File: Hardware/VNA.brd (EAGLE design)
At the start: 122 x 96 mm, 499 parts, among them IC1 ADL5801, IC10 LT5560, IC11 THS4521IDGKR, IC12 MCP33131D-10-E/MS, IC13 SI5351C, IC14 MAX2871, IC15 NCP702-3.3, IC16 RFSW6042, IC17 AP2114H, IC18 RFSW6042, IC19 MAX2871, IC2 LT5560, IC20 NCP702-3.3, IC21 AP2114H, IC22 QPC6324, IC23 RFSA3714, IC24 TRF37A73, IC25 QPC6324, IC26 QPC6324, IC27 QPC6324, IC28 LDL212PU50R, IC29 LDL212PU50R, IC3 THS4521IDGKR, IC30 LDL212PU50R, IC31 LDL212PU50R, IC32 TPS65265, IC34 NCP702-1.8, IC35 NCP702-1.8, IC36 NCP702-1.8, IC37 ADL5801, IC4 MCP33131D-10-E/MS, IC5 ADL5801, IC6 LT5560, IC7 THS4521IDGKR, IC8 MCP33131D-10-E/MS, IC9 STM32G431KB, J1 AMPHENOL_132289, J2 AMPHENOL_132289, J3 DCJ0202, J4 TYPE-C16P(073), Q1 FA-128 26MHz, T1 B012-617DB-1-63-B331, T2 B012-617DB-1-63-B331, T3 B012-617DB-1-63-B331, U2 6SLX9TQG144, U4 W25Q16BVSN, X4 DNP, X5 10MHz out, X6 10MHz in

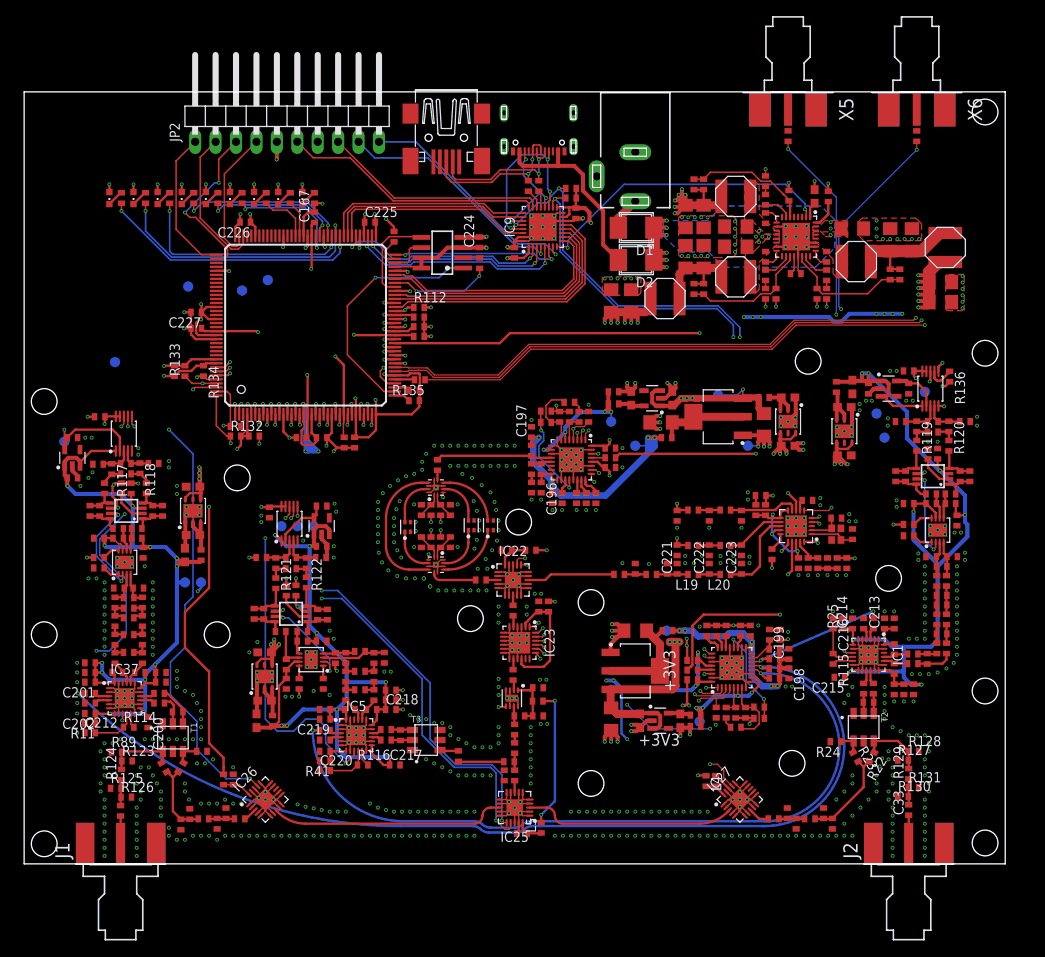
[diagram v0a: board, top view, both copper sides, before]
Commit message: Routing completed
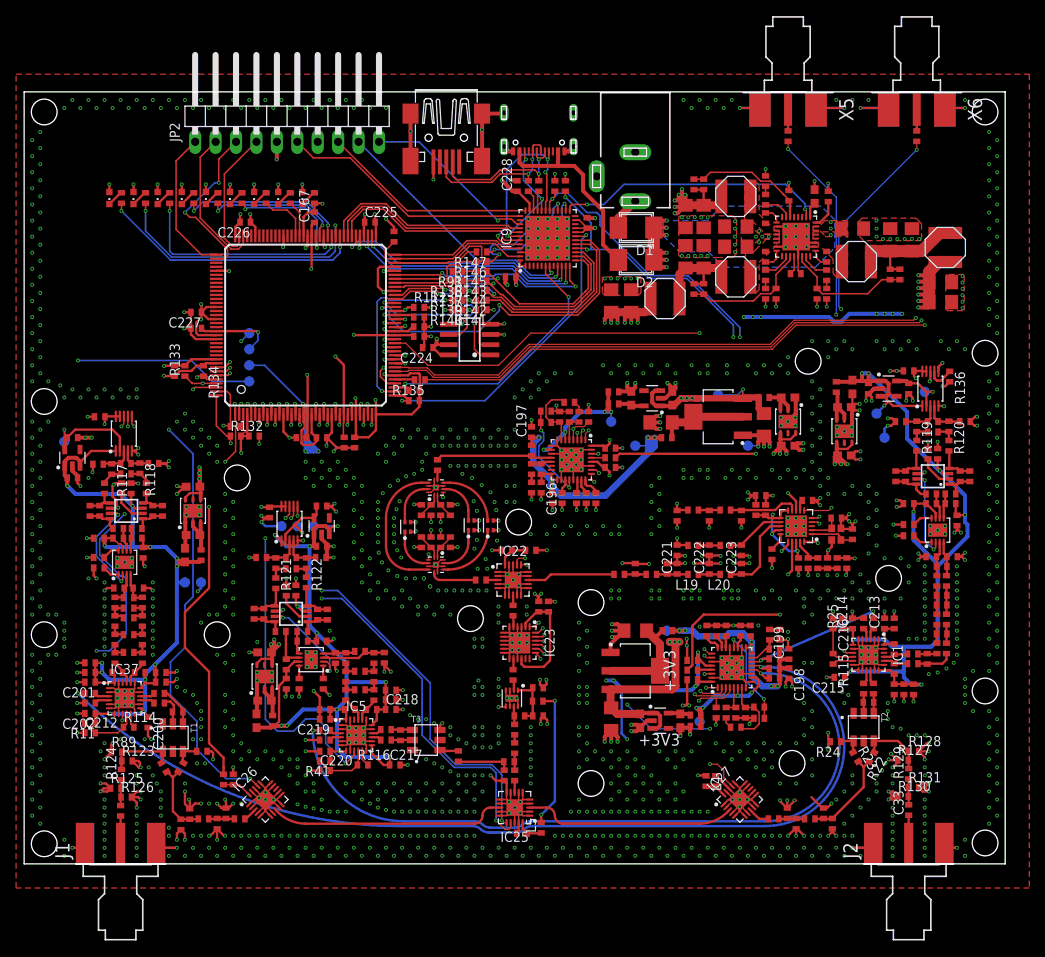
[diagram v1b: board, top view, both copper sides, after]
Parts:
- added C228: 100n, rcl:C0402
- added R137, R138, R139, R140, R141, R142, R143, R144, R145, R146, R147: 0, rcl:R0402
- IC9: value STM32G431KB -> STM32G431CB; device custom-ic:QFN50P500X500X100-33T345N -> custom-ic:QFN50P700X700X60-49T560N
- R91: value 22 -> 0
- moved TP5 16.9 mm to (28.0, 60.0)
- moved C224 14.6 mm to (50.2, 64.2), turned to 180 degrees
- moved TP3 12.4 mm to (28.0, 62.0)
- moved U4 11.3 mm to (55.4, 65.2)
- moved TP1 7.36 mm to (28.0, 64.0)
- moved TP6 6.99 mm to (28.0, 66.0)
- moved C192 3.04 mm to (60.5, 73.0), turned to 180 degrees
- moved R91 2.93 mm to (53.9, 73.7), turned to 180 degrees
- moved R95 2.02 mm to (66.0, 84.3), turned to 90 degrees
- moved C191 1.84 mm to (70.0, 79.7), turned to 90 degrees
- moved R90 1.66 mm to (67.3, 84.3), turned to 90 degrees
- moved IC9 1.52 mm to (65.1, 77.8)
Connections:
- removed net FLACH_MOSI: U2.P64, U4.5
- removed net FLASH_CLK: U2.P70, U4.6
- removed net FLASH_CS: U2.P38, U4.1
- removed net FLASH_MISO: R91.1, U4.2
- removed net MCU_NSS: IC9.9, U2.P67
- removed net N$190: IC9.24, JP2.6
- removed net N$191: IC9.23, JP2.8
- removed net N$194: R92.1, U2.P71
- removed net N$195: R93.1, U2.P39
- removed net N$196: R94.1, U2.P37
- new net FPGA_CCLK: R146.2, R91.2, U2.P70
- new net FPGA_CSO_B: R139.2, U2.P38
- new net FPGA_DIN: R138.2, R147.2, U2.P65
- new net FPGA_DONE: IC9.47, R92.1, U2.P71
- new net FPGA_INIT_B: IC9.6, R93.1, U2.P39
- new net FPGA_M1: R140.1, R141.2, U2.P60
- new net FPGA_MOSI: R137.2, U2.P64
- new net FPGA_PROGRAM_B: IC9.19, R94.1, U2.P37
- new net MCU_FLASH_CS: IC9.17, R142.1
- new net MCU_FPGA_CCLK: IC9.28, R146.1
- new net MCU_FPGA_DIN: IC9.26, R147.1
- new net MCU_FPGA_NSS: IC9.12, U2.P67
- new net N$237: R137.1, R144.2, U4.5
- new net N$240: R138.1, R143.2, U4.2
- new net N$241: R139.1, R142.2, U4.1
- new net SWCLK: IC9.37, JP2.6
- new net SWDIO: IC9.36, JP2.8
- net +3V3: now also C228.1, IC9.20, IC9.21, IC9.23, IC9.35, IC9.48, R141.1; no longer IC9.15, IC9.17
- net FPGA_RESET: now also IC9.45; no longer IC9.6
- net GND: now also C228.2, IC9.46, IC9.49, R140.2; no longer IC9.14, IC9.16, IC9.31, IC9.32, IC9.33, U2.P60
- net MCU_AUX1: now also IC9.9; no longer IC9.2
- net MCU_AUX2: now also IC9.10; no longer IC9.3
- net MCU_AUX3: now also IC9.11; no longer IC9.5
- net MCU_FPGA_UNUSED1: now also IC9.43; no longer IC9.30
- net MCU_FPGA_UNUSED2: now also IC9.41; no longer IC9.26
- net MCU_FPGA_UNUSED3: now also IC9.40; no longer IC9.25
- net MCU_INTR: now also IC9.18; no longer IC9.13
- net MCU_MISO: now also IC9.14, R143.1; no longer IC9.11
- net MCU_MOSI: now also IC9.15, R144.1; no longer IC9.12
- net MCU_SCK: now also IC9.13, R145.1; no longer IC9.10
- net N$187: now also IC9.33; no longer IC9.21
- net N$188: now also IC9.34; no longer IC9.22
- net N$192: now also IC9.7; no longer IC9.4
- net N$193: now also IC9.39; no longer IC9.7
- net N$197: now also R145.2, R91.1, U4.6; no longer R91.2, U2.P65
- net N$233: now also IC9.31, IC9.44; no longer IC9.19, IC9.29
- net N$234: now also IC9.32, IC9.42; no longer IC9.20, IC9.27
- net POWER_GOOD: now also IC9.25; no longer IC9.8
- net SCL: now also IC9.16; no longer IC9.18
- net SDA: now also IC9.30; no longer IC9.28
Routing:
- net GND: track 451.3 -> 746.5 mm, vias 785 -> 1555
- net FPGA_PROGRAM_B: track 0.00 -> 40.4 mm, vias 0 -> 2
- net FPGA_INIT_B: track 0.00 -> 33.3 mm, vias 0 -> 2
- net N$190: track 32.5 -> 0.00 mm
- net SWCLK: track 0.00 -> 31.5 mm
- net FLASH_CS: track 30.2 -> 0.00 mm, vias 2 -> 0
- net MCU_NSS: track 29.4 -> 0.00 mm
- net N$191: track 28.1 -> 0.00 mm
- net SWDIO: track 0.00 -> 26.8 mm
- net MCU_FPGA_NSS: track 0.00 -> 26.3 mm, vias 0 -> 2
- net MCU_FLASH_CS: track 0.00 -> 23.4 mm
- net FPGA_CSO_B: track 0.00 -> 22.7 mm, vias 0 -> 2
- net N$163: track 85.0 -> 107.4 mm, vias 18 -> 19
- net FPGA_DONE: track 0.00 -> 20.7 mm
- net FPGA_CCLK: track 0.00 -> 17.8 mm
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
